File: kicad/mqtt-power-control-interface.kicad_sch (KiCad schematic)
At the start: 16 parts, among them J1 Conn_01x04_Pin, J2 Conn_01x04_Pin, J3 Conn_01x04_Pin, J4 Conn_01x04_Pin, J5 Conn_01x04_Pin, J6 Conn_01x04_Pin, U1 LTV-847, U2 LTV-847, U3 LTV-847, U4 RPi Pico W

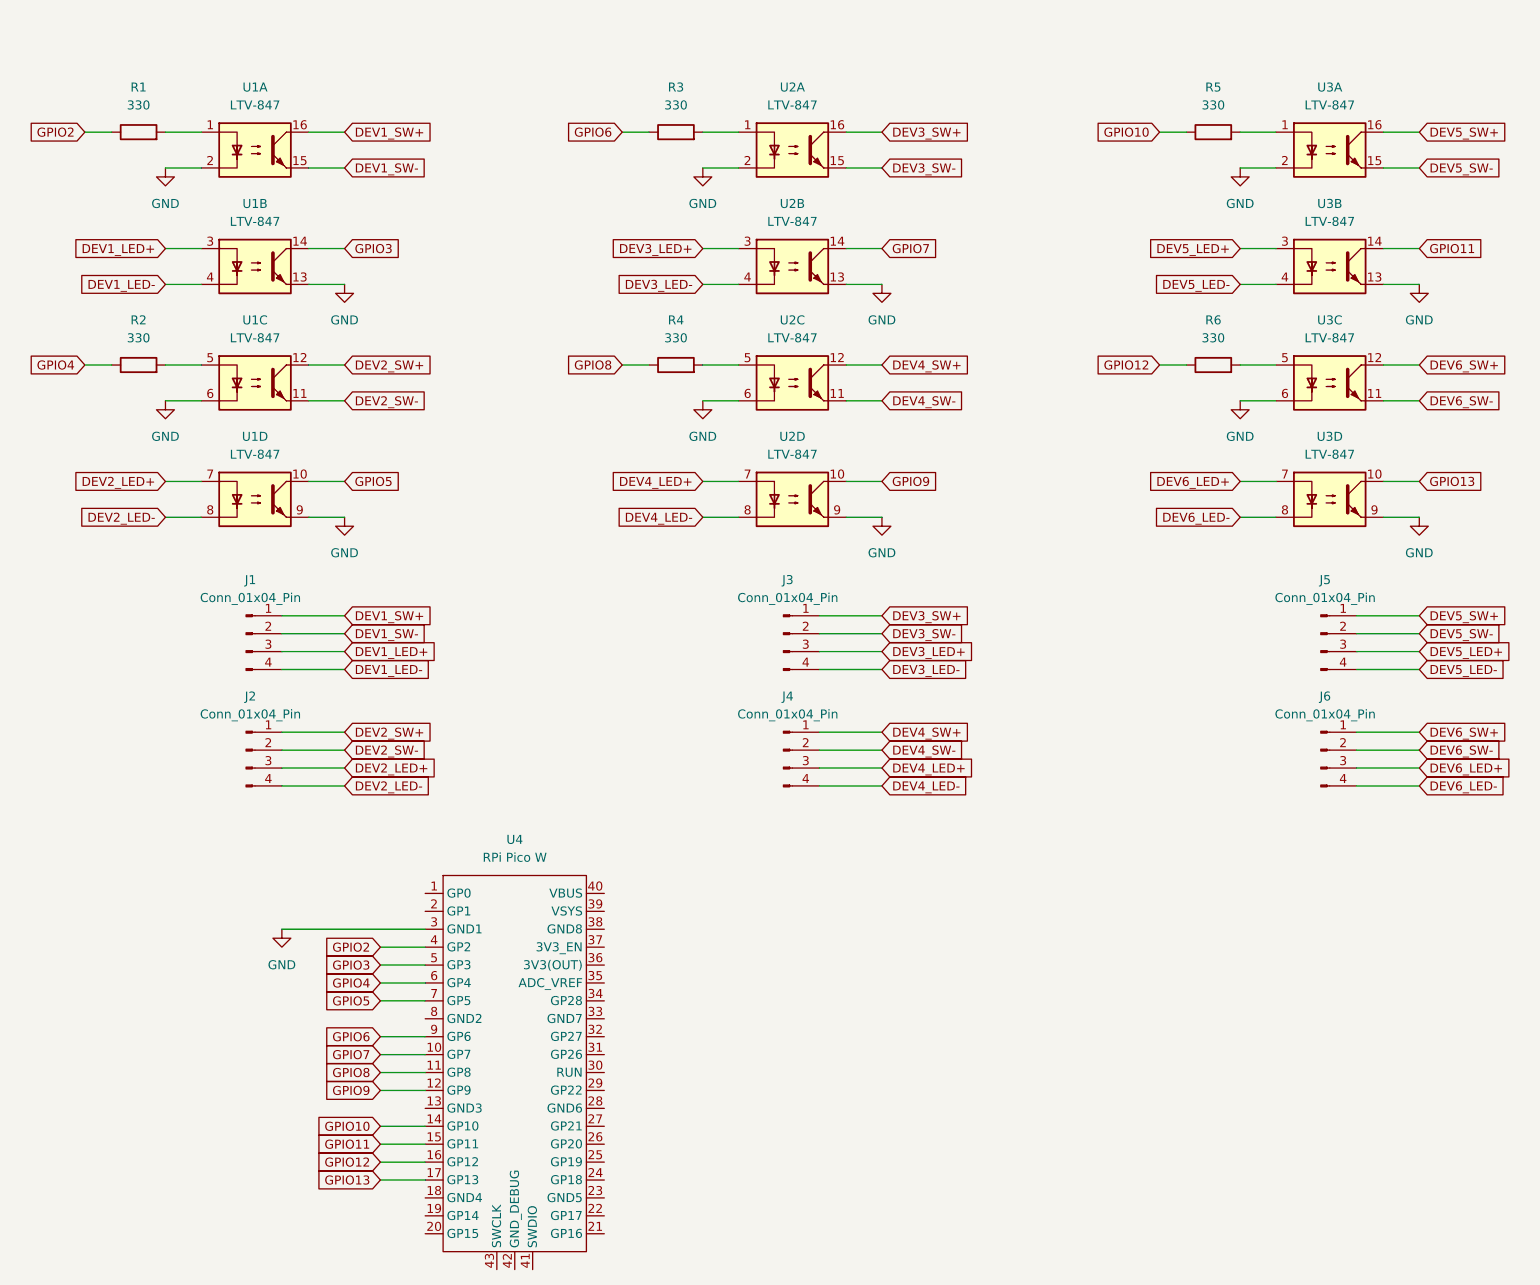
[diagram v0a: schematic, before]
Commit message: Enhanced schematic and board
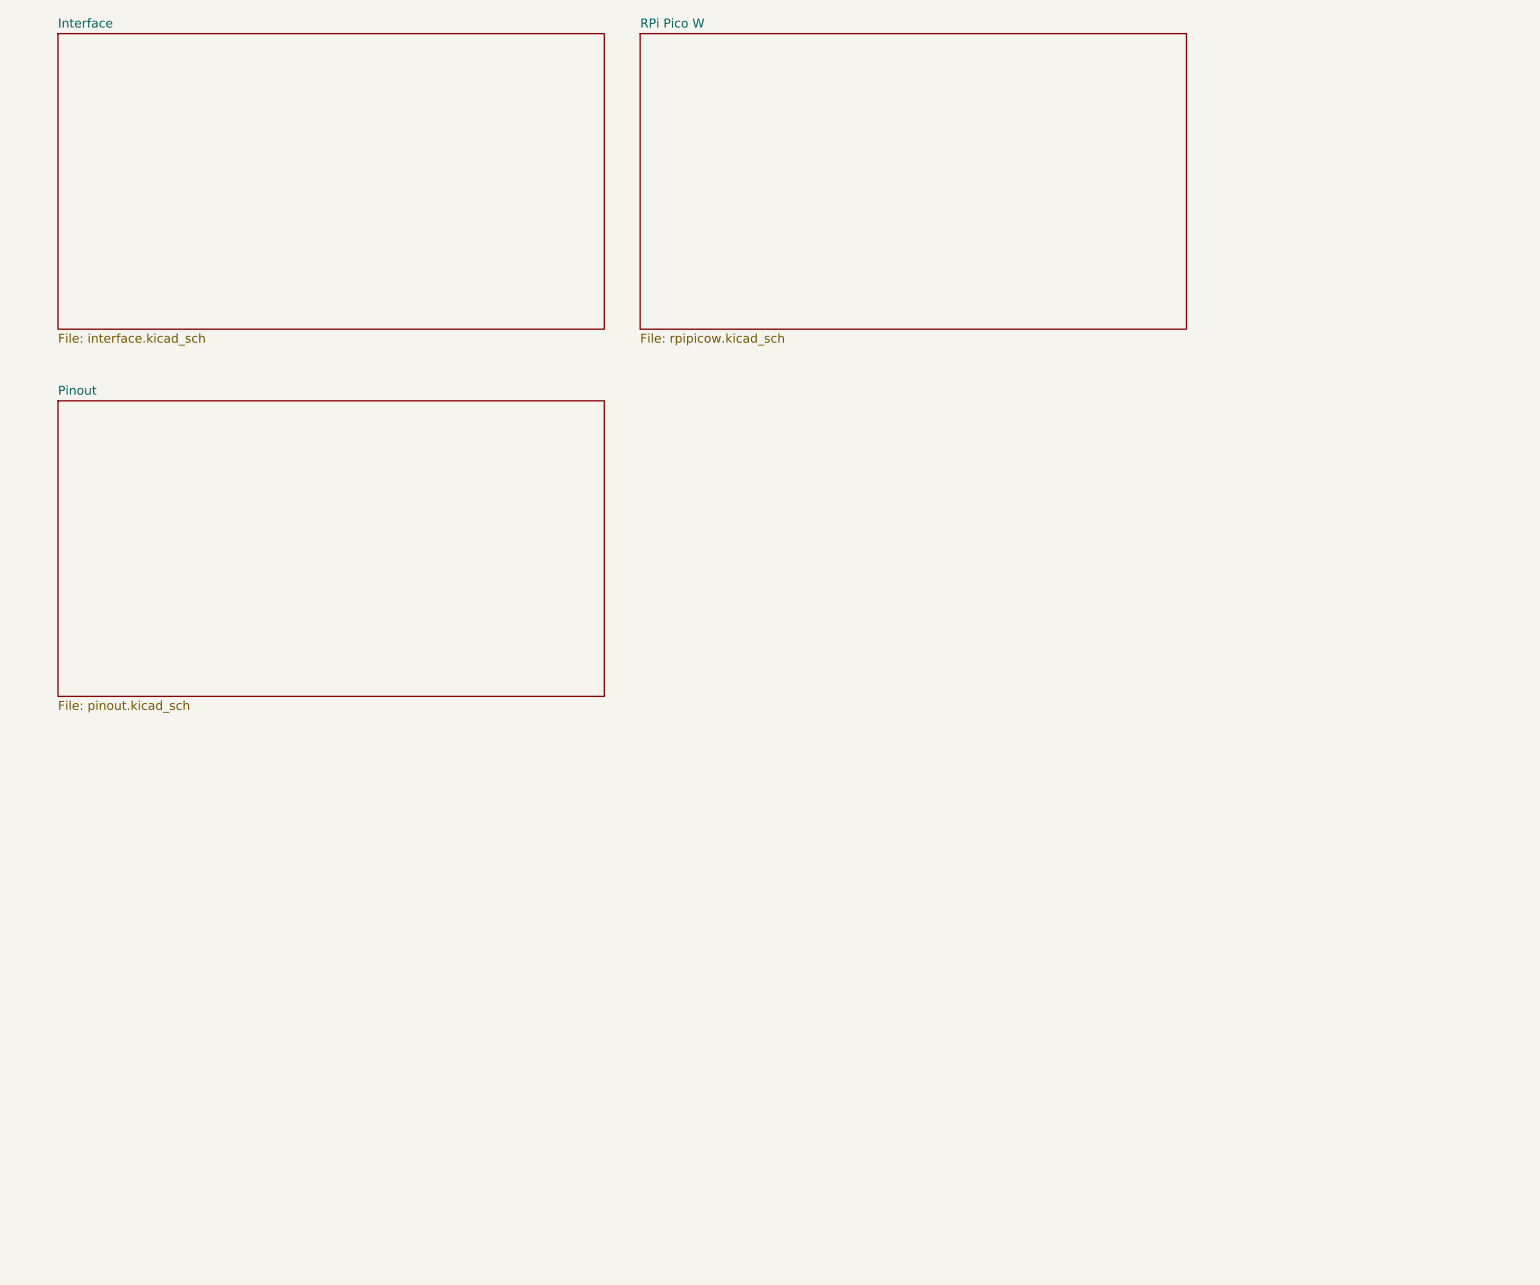
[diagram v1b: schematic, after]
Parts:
- removed J1, J2, J3, J4, J5, J6: Conn_01x04_Pin, Connector_Molex:Molex_KK-254_AE-6410-04A_1x04_P2.54mm_Vertical, symbol Connector:Conn_01x04_Pin
- removed R1, R2, R3, R4, R5, R6: 330, Resistor_THT:R_Axial_DIN0204_L3.6mm_D1.6mm_P7.62mm_Horizontal, symbol Device:R
- removed U1, U2, U3: LTV-847, Package_DIP:DIP-16_W7.62mm, symbol Isolator:LTV-847
- removed U4: RPi Pico W, Custom:RPI Pico W, symbol Custom:RPi Pico W
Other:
- added sheet Interface (interface.kicad_sch)
- added sheet Pinout (pinout.kicad_sch)
- added sheet RPi Pico W (rpipicow.kicad_sch)
- title: (none) -> mqtt-power-control-interface
